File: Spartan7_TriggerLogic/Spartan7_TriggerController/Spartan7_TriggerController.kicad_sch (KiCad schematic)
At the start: 0 parts

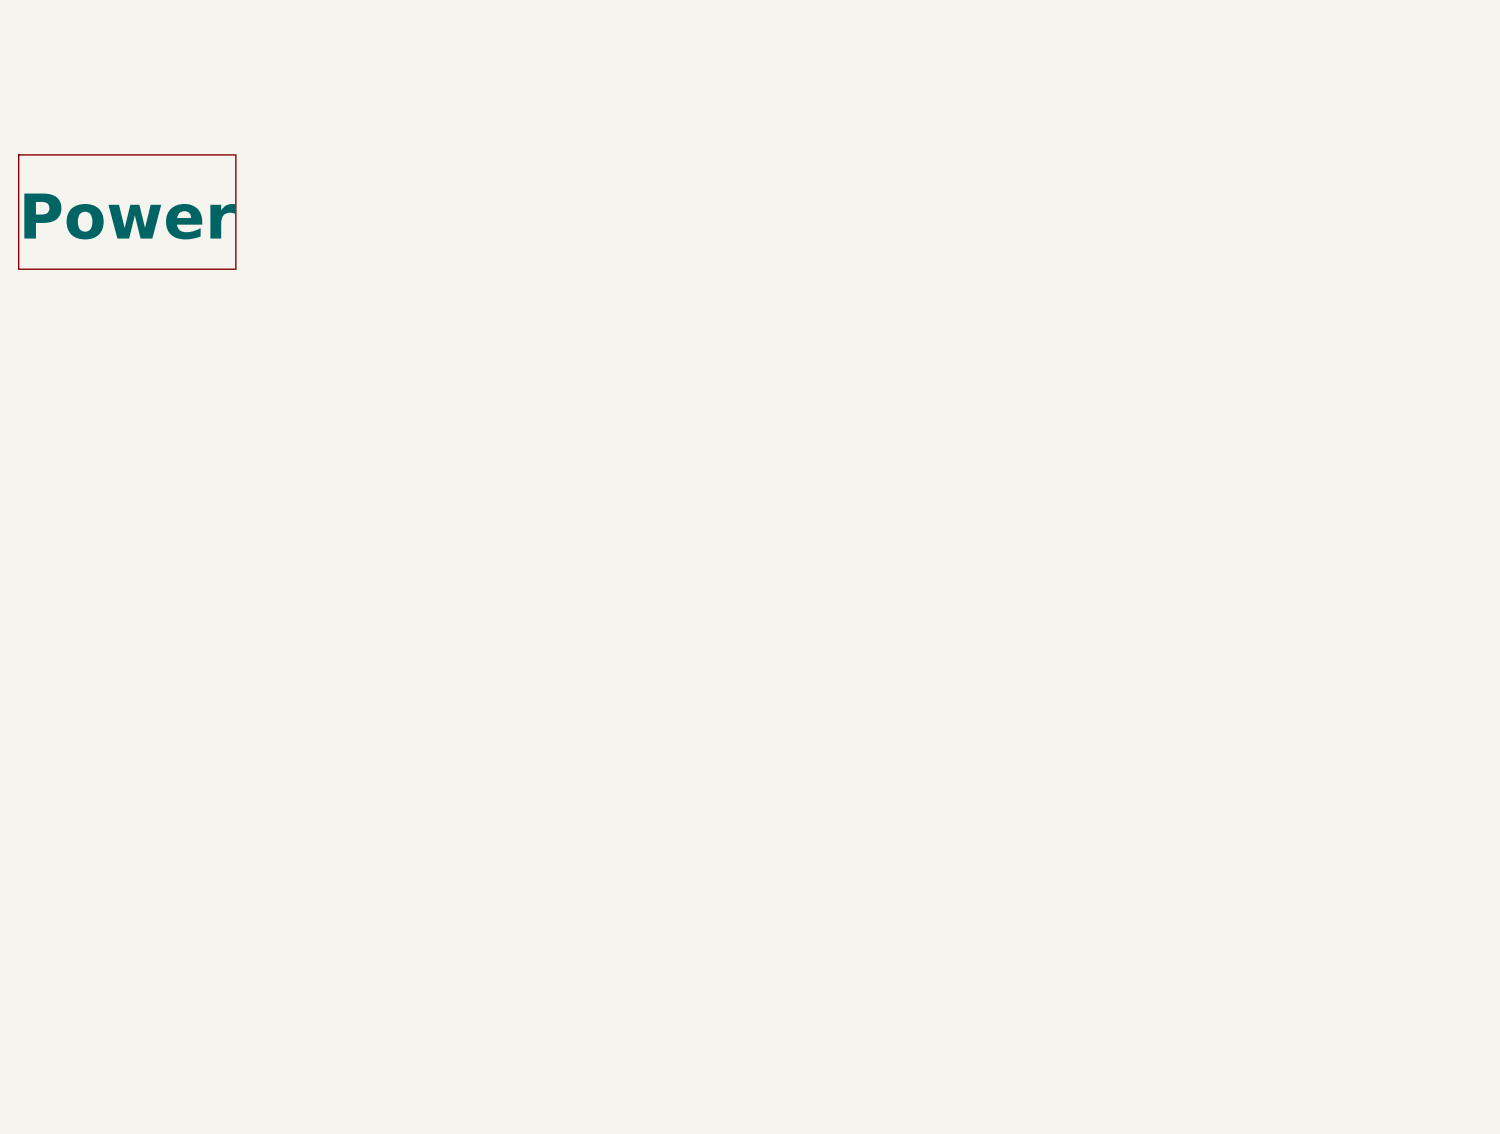
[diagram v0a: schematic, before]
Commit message: .
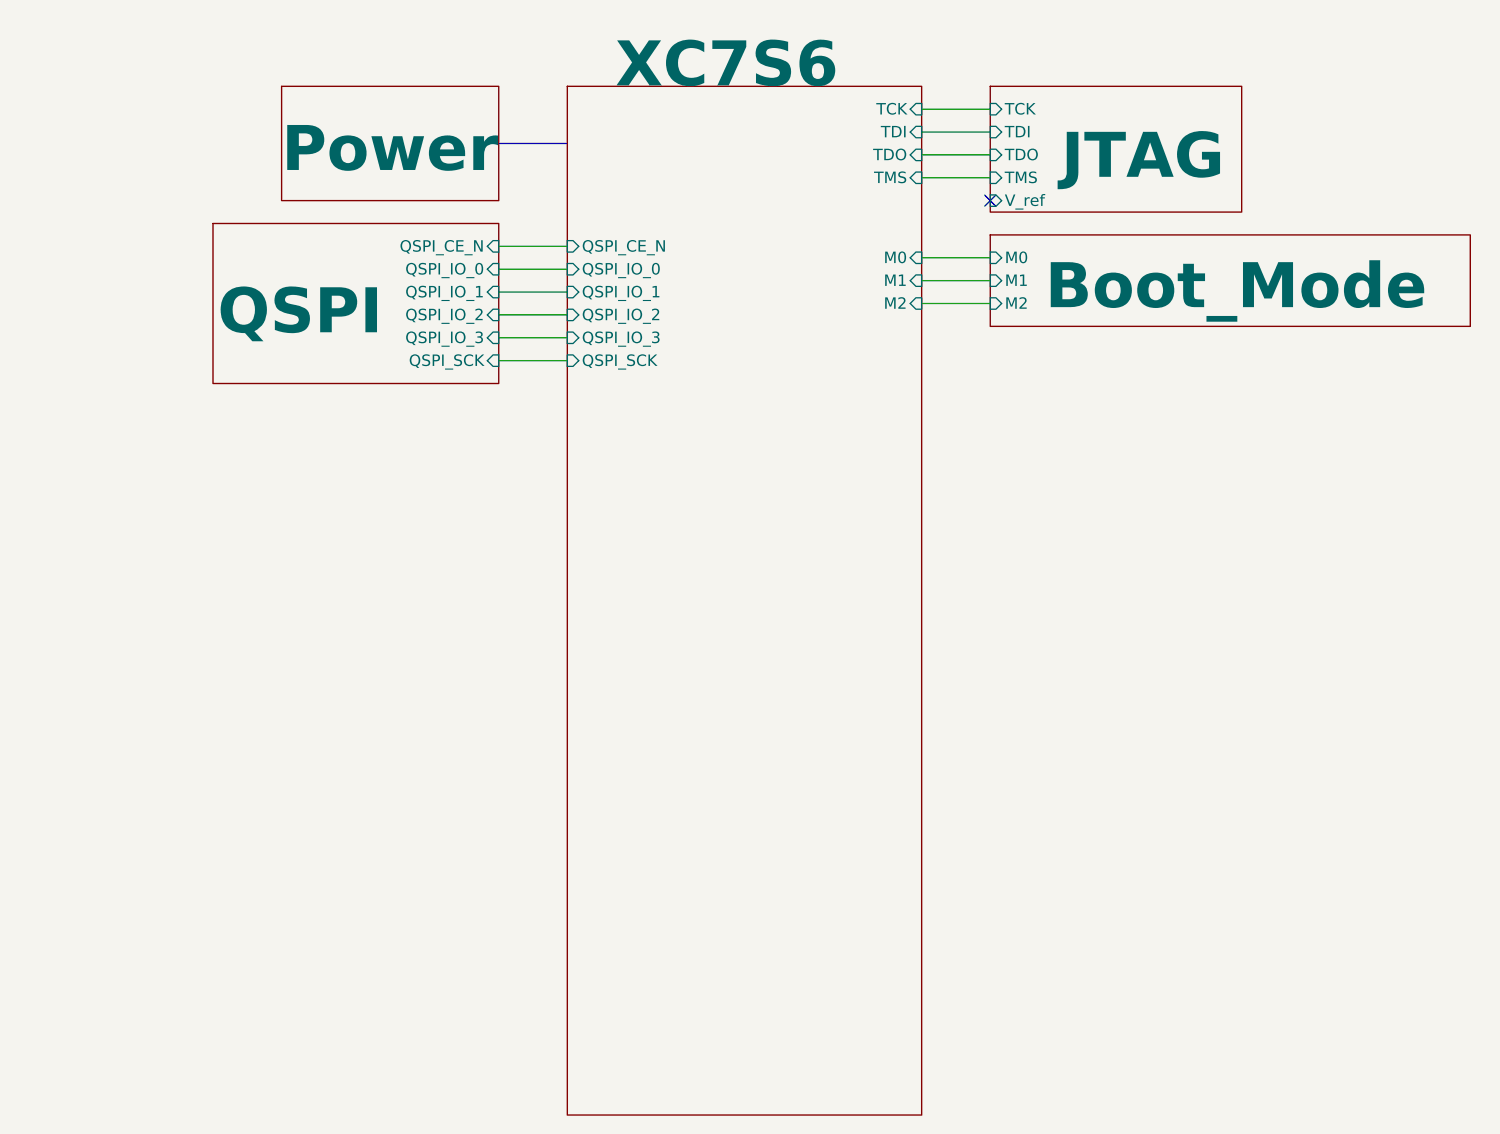
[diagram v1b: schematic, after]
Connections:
- no-connect marks 0 -> 1
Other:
- added sheet Boot_Mode (Boot_Mode.kicad_sch)
- added sheet JTAG (JTAG.kicad_sch)
- added sheet QSPI (QSPI_IS25LP256D.kicad_sch)
- added sheet XC7S6 (XC7S6_FTGB196.kicad_sch)
